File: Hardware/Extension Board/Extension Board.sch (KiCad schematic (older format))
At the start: 5 parts, among them J1 ARDUINO_DIGITAL, J2 ARDUINO_COMMS, J3 ARDUINO_ANALOG

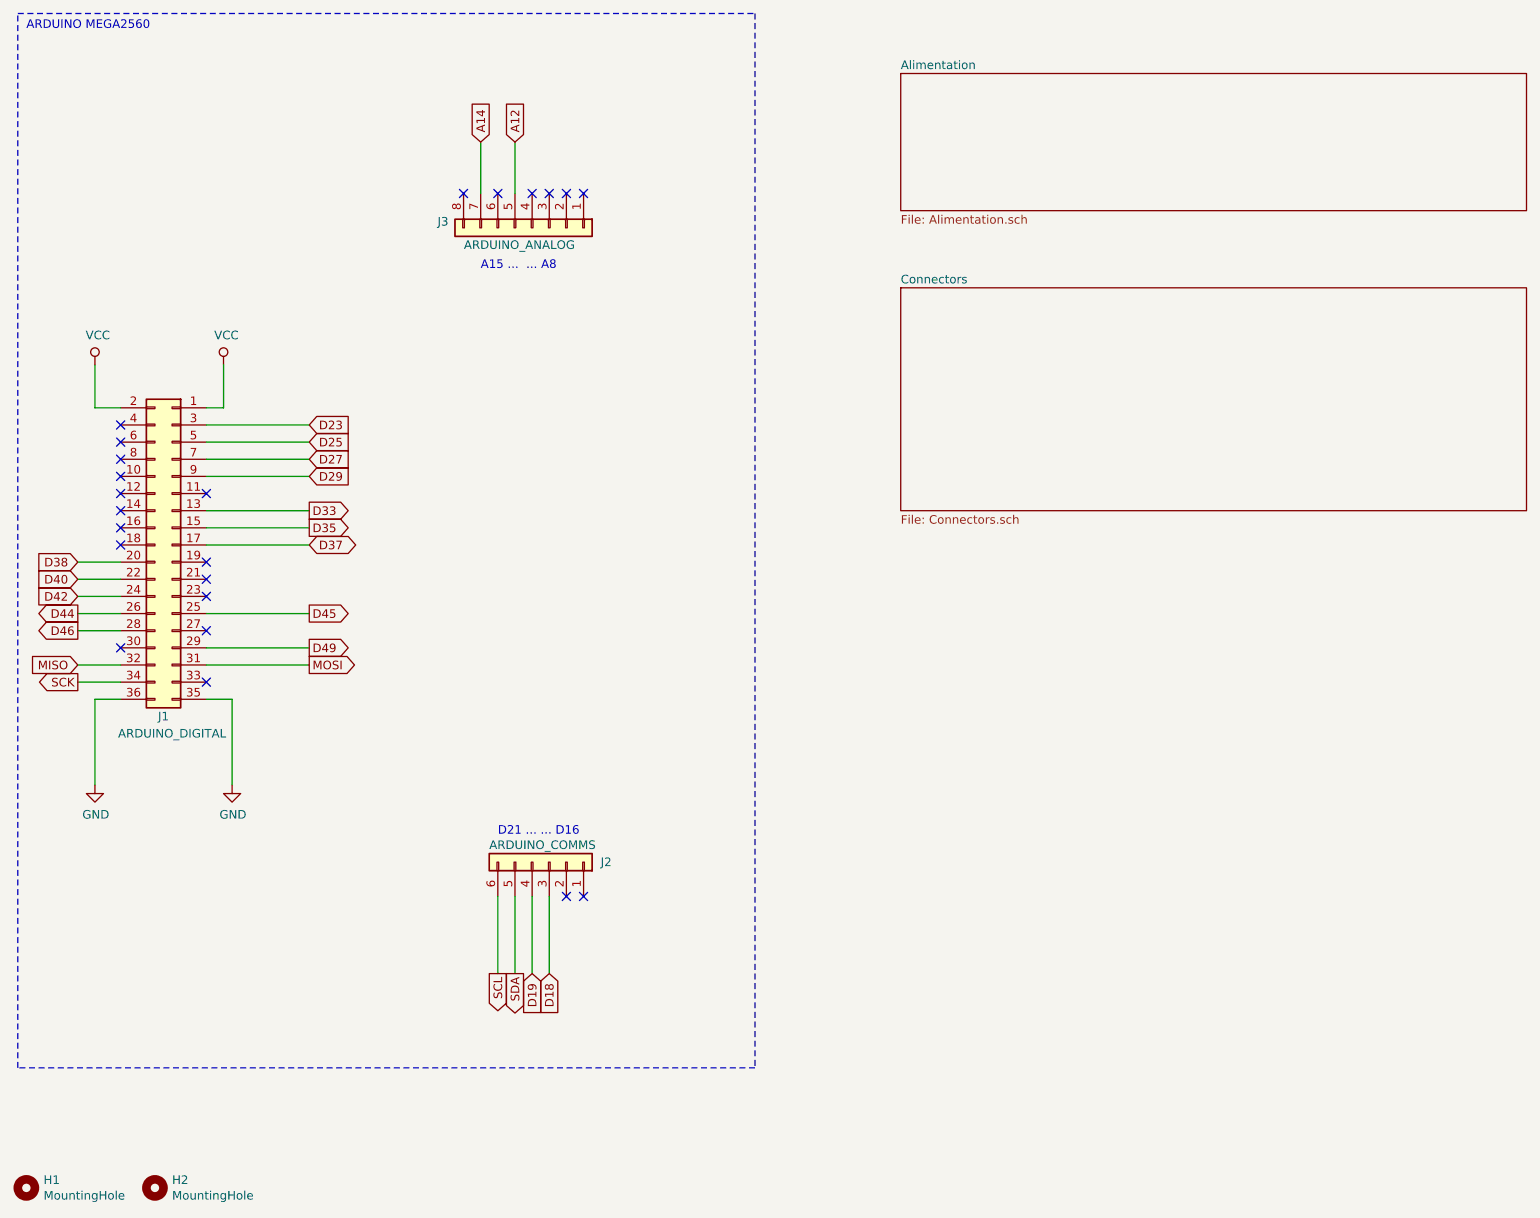
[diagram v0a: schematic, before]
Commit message: Design carte extension
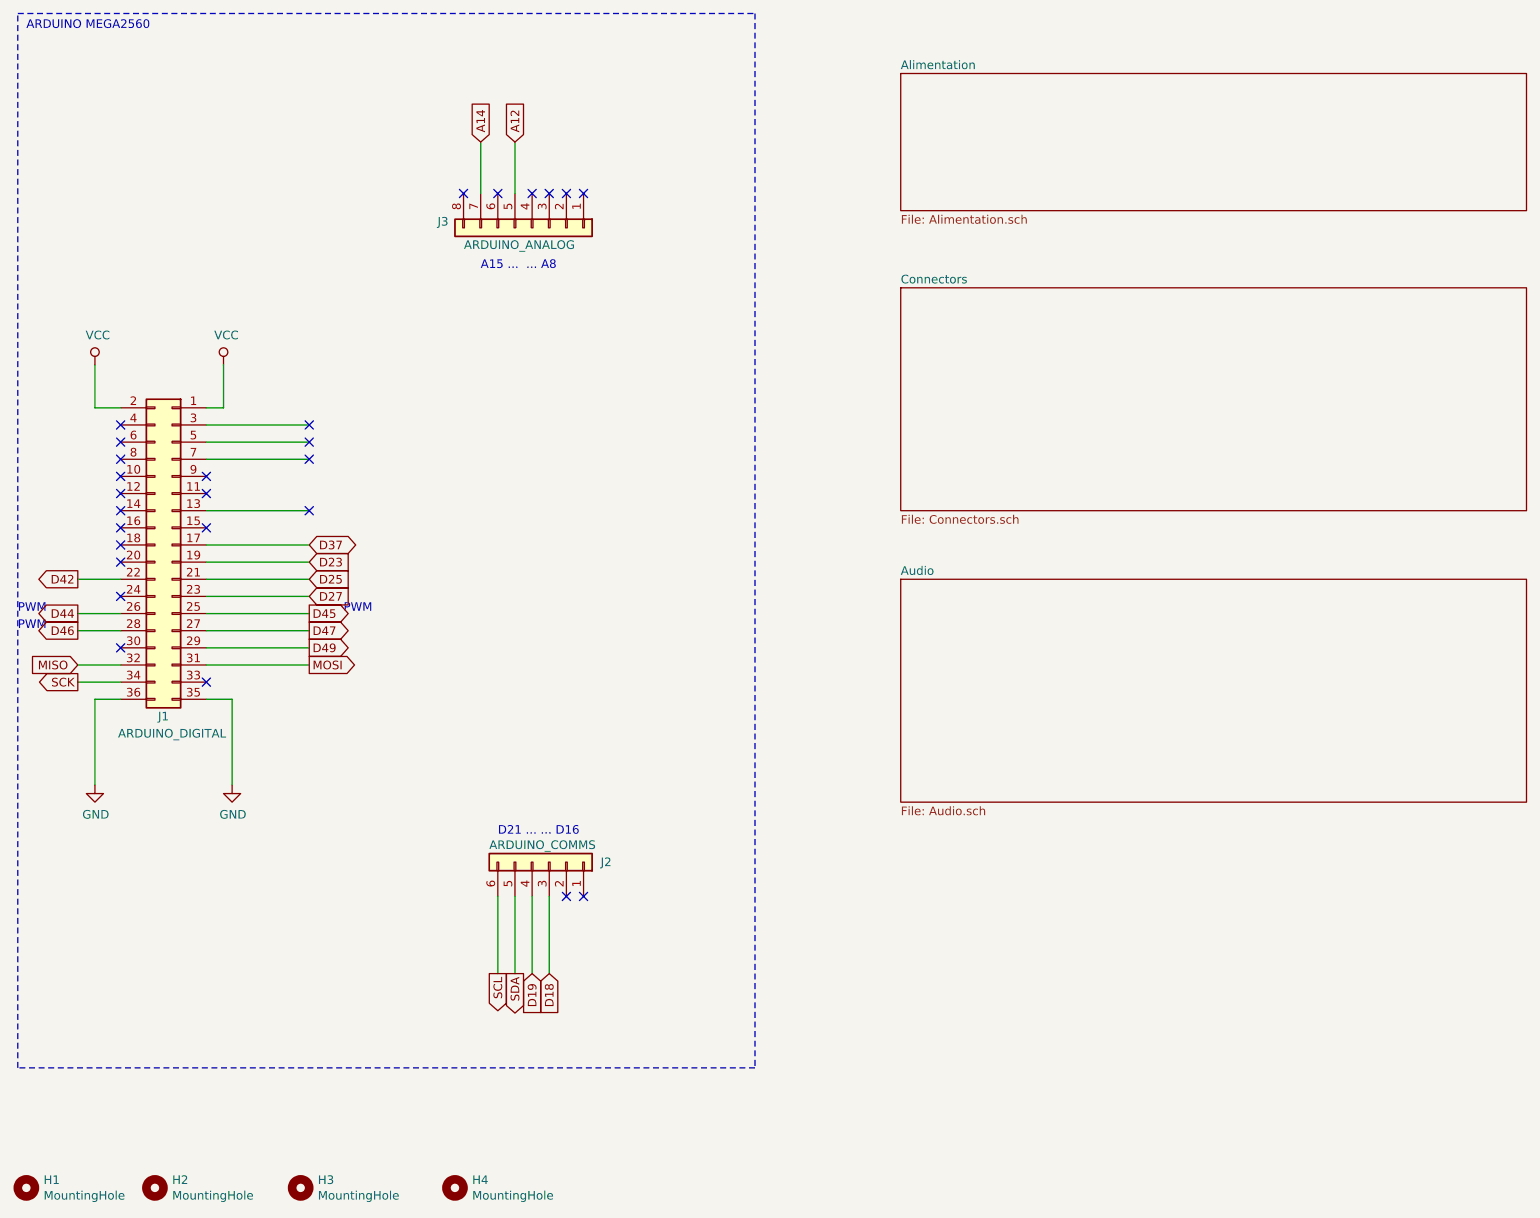
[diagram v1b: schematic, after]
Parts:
- added H3, H4: MountingHole, MountingHole:MountingHole_3.2mm_M3, symbol Mechanical:MountingHole
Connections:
- net D40 is gone; now on net D42: J1.22 (Pin_22)
- net D23: now also J1.19 (Pin_19); no longer J1.3 (Pin_3)
- net D25: now also J1.21 (Pin_21); no longer J1.5 (Pin_5)
- net D27: now also J1.23 (Pin_23); no longer J1.7 (Pin_7)
- net D42: no longer J1.24 (Pin_24)
- net D47: now reaches J1.27 (Pin_27)
- net D29: no longer names the net of J1.9 (Pin_9)
- net D33: no longer names the net of J1.13 (Pin_13)
- net D35: no longer names the net of J1.15 (Pin_15)
- net D38: no longer names the net of J1.20 (Pin_20)
- no-connect marks 23 -> 27
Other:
- note added: "PWM"
- note added: "PWM\n"
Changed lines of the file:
@@
 $Descr A4 11693 8268
 encoding utf-8
-Sheet 1 3
+Sheet 1 4
 Title "Durcretet L.024 : Extension Board"
 Date "2022-04-02"
@@
 	0    1    1    0
 $EndComp
-Wire Wire Line
-	1800 3300 2400 3300
 Wire Wire Line
 	1800 3500 2400 3500
@@
 Wire Wire Line
 	3600 1650 3600 1350
-Text GLabel 2400 3500 2    50   Output ~ 0
-D33
+Text GLabel 1050 3900 0    50   Output ~ 0
+D42
 Wire Wire Line
 	1800 3000 2400 3000
 Wire Wire Line
 	1800 3100 2400 3100
-Wire Wire Line
-	1800 4300 2400 4300
-Text GLabel 2400 4100 2    50   Output ~ 0
-D45
-Wire Wire Line
-	1800 4100 2400 4100
+Text GLabel 2400 4300 2    50   Output ~ 0
+D49
 Wire Wire Line
 	1800 3200 2400 3200
@@
 Text GLabel 1050 4200 0    50   Output ~ 0
 D46
-NoConn ~ 1800 3800
-NoConn ~ 1800 4200
-Text GLabel 2400 3200 2    50   Input ~ 0
+Text GLabel 2400 4000 2    50   Input ~ 0
 D27
-Text GLabel 2400 3100 2    50   Input ~ 0
+Text GLabel 2400 3900 2    50   Input ~ 0
 D25
-Text GLabel 2400 3000 2    50   Input ~ 0
+Text GLabel 2400 3800 2    50   Input ~ 0
 D23
+$Comp
+L Connector_Generic:Conn_01x06 J2
+U 1 1 5EEEB64E
+P 3800 5550
+F 0 "J2" V 3800 5850 50  0000 L CNN
+F 1 "ARDUINO_COMMS" V 3900 5200 50  0000 L CNN
+F 2 "Connector_PinHeader_2.54mm:PinHeader_1x06_P2.54mm_Vertical" H 3800 5550 50  0001 C CNN
+F 3 "~" H 3800 5550 50  0001 C CNN
+	1    3800 5550
+	0    1    -1   0
+$EndComp
+$Comp
+L Mechanical:MountingHole H1
+U 1 1 5EF76CE6
+P 750 7450
+F 0 "H1" H 850 7496 50  0000 L CNN
+F 1 "MountingHole" H 850 7405 50  0000 L CNN
+F 2 "MountingHole:MountingHole_3.2mm_M3" H 750 7450 50  0001 C CNN
+F 3 "~" H 750 7450 50  0001 C CNN
+	1    750  7450
+	1    0    0    -1
+$EndComp
+$Comp
+L Mechanical:MountingHole H2
+U 1 1 5EF77663
+P 1500 7450
+F 0 "H2" H 1600 7496 50  0000 L CNN
+F 1 "MountingHole" H 1600 7405 50  0000 L CNN
+F 2 "MountingHole:MountingHole_3.2mm_M3" H 1500 7450 50  0001 C CNN
+F 3 "~" H 1500 7450 50  0001 C CNN
+	1    1500 7450
+	1    0    0    -1
+$EndComp
+NoConn ~ 1300 4300
+NoConn ~ 1300 3700
+Wire Wire Line
+	1050 4100 1300 4100
+Wire Wire Line
+	1050 4200 1300 4200
+Wire Wire Line
+	1050 4400 1300 4400
+Wire Wire Line
+	1050 4500 1300 4500
+Wire Wire Line
+	1150 4600 1300 4600
+NoConn ~ 1300 3500
+Wire Wire Line
+	1150 2900 1300 2900
+NoConn ~ 1300 3600
+NoConn ~ 1800 3400
+Text Notes 3400 2100 0    50   ~ 0
+A15 ...  ... A8
+Text Notes 3500 5400 0    50   ~ 0
+D21 ... ... D16
+NoConn ~ 4000 5750
+NoConn ~ 3900 5750
+$Comp
+L power:GND #PWR0106
+U 1 1 6247305B
+P 1950 5100
+F 0 "#PWR0106" H 1950 4850 50  0001 C CNN
+F 1 "GND" H 1955 4927 50  0000 C CNN
+F 2 "" H 1950 5100 50  0001 C CNN
+F 3 "" H 1950 5100 50  0001 C CNN
+	1    1950 5100
+	1    0    0    -1
+$EndComp
+Wire Wire Line
+	1150 4600 1150 5100
+Wire Wire Line
+	1950 4600 1950 5100
+$Comp
+L power:VCC #PWR0107
+U 1 1 6247ECAC
+P 1900 2650
+F 0 "#PWR0107" H 1900 2500 50  0001 C CNN
+F 1 "VCC" H 1917 2823 50  0000 C CNN
+F 2 "" H 1900 2650 50  0001 C CNN
+F 3 "" H 1900 2650 50  0001 C CNN
+	1    1900 2650
+	1    0    0    -1
+$EndComp
+Wire Wire Line
+	1900 2650 1900 2900
+Wire Wire Line
+	1150 2650 1150 2900
+Text GLabel 3800 6200 3    50   Input ~ 0
+D18
+Text GLabel 3700 6200 3    50   Input ~ 0
+D19
+Wire Wire Line
+	3700 5750 3700 6200
+Wire Wire Line
+	3800 5750 3800 6200
+Text GLabel 2400 3700 2    50   BiDi ~ 0
+D37
+Wire Wire Line
+	1800 3700 2400 3700
+$Sheet
+S 5850 950  3650 800
+U 624BFCA3
+F0 "Alimentation" 50
+F1 "Alimentation.sch" 50
+$EndSheet
+Text GLabel 2400 4100 2    50   Output ~ 0
+D45
+$Sheet
+S 5850 2200 3650 1300
+U 624DD375
+F0 "Connectors" 50
+F1 "Connectors.sch" 50
+$EndSheet
+$Sheet
+S 5850 3900 3650 1300
+U 6250A423
+F0 "Audio" 50
+F1 "Audio.sch" 50
+$EndSheet
+NoConn ~ 1800 3300
+NoConn ~ 1300 3800
+NoConn ~ 1300 4000
+$Comp
+L Mechanical:MountingHole H3
+U 1 1 62559996
+P 2350 7450
+F 0 "H3" H 2450 7496 50  0000 L CNN
+F 1 "MountingHole" H 2450 7405 50  0000 L CNN
+F 2 "MountingHole:MountingHole_3.2mm_M3" H 2350 7450 50  0001 C CNN
+F 3 "~" H 2350 7450 50  0001 C CNN
+	1    2350 7450
+	1    0    0    -1
+$EndComp
+$Comp
+L Mechanical:MountingHole H4
+U 1 1 62559CD8
+P 3250 7450
+F 0 "H4" H 3350 7496 50  0000 L CNN
+F 1 "MountingHole" H 3350 7405 50  0000 L CNN
+F 2 "MountingHole:MountingHole_3.2mm_M3" H 3250 7450 50  0001 C CNN
+F 3 "~" H 3250 7450 50  0001 C CNN
+	1    3250 7450
+	1    0    0    -1
+$EndComp
+NoConn ~ 1800 3600
+Wire Wire Line
+	1800 4200 2400 4200
+Wire Wire Line
+	2400 4300 1800 4300
+Wire Wire Line
+	2400 4100 1800 4100
 $Comp
 L Connector_Generic:Conn_02x18_Odd_Even J1
@@
 	-1   0    0    -1
 $EndComp
-Text GLabel 2400 3300 2    50   Input ~ 0
-D29
-$Comp
-L Connector_Generic:Conn_01x06 J2
-U 1 1 5EEEB64E
-P 3800 5550
-F 0 "J2" V 3800 5850 50  0000 L CNN
-F 1 "ARDUINO_COMMS" V 3900 5200 50  0000 L CNN
-F 2 "Connector_PinHeader_2.54mm:PinHeader_1x06_P2.54mm_Vertical" H 3800 5550 50  0001 C CNN
-F 3 "~" H 3800 5550 50  0001 C CNN
-	1    3800 5550
-	0    1    -1   0
-$EndComp
-Text GLabel 1050 4000 0    50   Input ~ 0
-D42
-Text GLabel 1050 3900 0    50   Input ~ 0
-D40
-NoConn ~ 1800 3900
-$Comp
-L Mechanical:MountingHole H1
-U 1 1 5EF76CE6
-P 750 7450
-F 0 "H1" H 850 7496 50  0000 L CNN
-F 1 "MountingHole" H 850 7405 50  0000 L CNN
-F 2 "MountingHole:MountingHole_3.2mm_M3" H 750 7450 50  0001 C CNN
-F 3 "~" H 750 7450 50  0001 C CNN
-	1    750  7450
-	1    0    0    -1
-$EndComp
-$Comp
-L Mechanical:MountingHole H2
-U 1 1 5EF77663
-P 1500 7450
-F 0 "H2" H 1600 7496 50  0000 L CNN
-F 1 "MountingHole" H 1600 7405 50  0000 L CNN
-F 2 "MountingHole:MountingHole_3.2mm_M3" H 1500 7450 50  0001 C CNN
-F 3 "~" H 1500 7450 50  0001 C CNN
-	1    1500 7450
-	1    0    0    -1
-$EndComp
-NoConn ~ 1800 4000
-NoConn ~ 1300 4300
-NoConn ~ 1300 3700
-Wire Wire Line
-	1050 4000 1300 4000
+Text GLabel 2400 4200 2    50   Output ~ 0
+D47
+Text Notes 2600 4100 0    50   ~ 0
+PWM
+Text Notes 700  4100 0    50   ~ 0
+PWM\n
+Text Notes 700  4200 0    50   ~ 0
+PWM
 Wire Wire Line
 	1050 3900 1300 3900
-Wire Wire Line
-	1050 4100 1300 4100
-Wire Wire Line
-	1050 4200 1300 4200
-Wire Wire Line
-	1050 4400 1300 4400
-Wire Wire Line
-	1050 4500 1300 4500
-Wire Wire Line
-	1150 4600 1300 4600
-NoConn ~ 1300 3500
-Wire Wire Line
-	1150 2900 1300 2900
-NoConn ~ 1300 3600
-Wire Wire Line
-	1300 3800 1050 3800
-NoConn ~ 1800 3400
-Text GLabel 1050 3800 0    50   Input ~ 0
-D38
-Text Notes 3400 2100 0    50   ~ 0
-A15 ...  ... A8
-Text Notes 3500 5400 0    50   ~ 0
-D21 ... ... D16
-NoConn ~ 4000 5750
-NoConn ~ 3900 5750
-$Comp
-L power:GND #PWR0106
-U 1 1 6247305B
-P 1950 5100
-F 0 "#PWR0106" H 1950 4850 50  0001 C CNN
-F 1 "GND" H 1955 4927 50  0000 C CNN
-F 2 "" H 1950 5100 50  0001 C CNN
-F 3 "" H 1950 5100 50  0001 C CNN
-	1    1950 5100
-	1    0    0    -1
-$EndComp
-Wire Wire Line
-	1150 4600 1150 5100
-Wire Wire Line
-	1950 4600 1950 5100
-$Comp
-L power:VCC #PWR0107
-U 1 1 6247ECAC
-P 1900 2650
-F 0 "#PWR0107" H 1900 2500 50  0001 C CNN
-F 1 "VCC" H 1917 2823 50  0000 C CNN
-F 2 "" H 1900 2650 50  0001 C CNN
-F 3 "" H 1900 2650 50  0001 C CNN
-	1    1900 2650
-	1    0    0    -1
-$EndComp
-Wire Wire Line
-	1900 2650 1900 2900
-Wire Wire Line
-	1150 2650 1150 2900
-Text GLabel 3800 6200 3    50   Input ~ 0
-D18
-Text GLabel 3700 6200 3    50   Input ~ 0
-D19
-Wire Wire Line
-	3700 5750 3700 6200
-Wire Wire Line
-	3800 5750 3800 6200
-Text GLabel 2400 3600 2    50   Output ~ 0
-D35
-Wire Wire Line
-	1800 3600 2400 3600
-Text GLabel 2400 3700 2    50   BiDi ~ 0
-D37
-Wire Wire Line
-	1800 3700 2400 3700
-$Sheet
-S 5850 950  3650 800
-U 624BFCA3
-F0 "Alimentation" 50
-F1 "Alimentation.sch" 50
-$EndSheet
-Text GLabel 2400 4300 2    50   Output ~ 0
-D49
-$Sheet
-S 5850 2200 3650 1300
-U 624DD375
-F0 "Connectors" 50
-F1 "Connectors.sch" 50
-$EndSheet
+NoConn ~ 2400 3500
+NoConn ~ 2400 3000
+NoConn ~ 2400 3100
+NoConn ~ 2400 3200
+Wire Wire Line
+	1800 3800 2400 3800
+Wire Wire Line
+	1800 3900 2400 3900
+Wire Wire Line
+	1800 4000 2400 4000
 $EndSCHEMATC
